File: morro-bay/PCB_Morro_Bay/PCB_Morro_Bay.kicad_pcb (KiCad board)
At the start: 2 copper layers, 220 x 145.5 mm, 346 parts, among them J1 POWER, J10 5V_12_8, J11 5V_12_9, J12 5V_12_10, J13 5V_12_11, J14 5V_12_12, J15 5V_12_13, J16 5V_12_14, J17 10V_12_1, J18 10V_12_2, J19 10V_12_3, J2 CAN, J20 10V_12_4, J21 10V_12_5, J22 10V_12_6, J23 POWER_OUT, J24 5V_16_1, J25 5V_16_2, J26 5V_16_3, J27 5V_16_4, J28 10V_16_1, J29 10V_16_2, J3 5V_12_1, J30 10V_16_3, J31 10V_16_4, J32 5V_16_5, J33 5V_16_6, J34 5V_16_7, J35 5V_16_8, J36 SWD, J37 GPIO, J38 USB_B, J39 ESERCOM, J4 5V_12_2, J5 5V_12_3, J6 5V_12_4, J7 5V_12_5, J8 5V_12_6, J9 5V_12_7, SW1 INPUT_RANGE_SEL_1, SW2 INPUT_RANGE_SEL_2, SW3 RESET, SW4 INPUT_RANGE_SEL_3, U1 MCP2515-xSO, U10 LM2902, U11 LM2902, U12 LM2902, U13 V7805-2000R, U2 SN65HVD232, U26 ADS114S08BIPBSR, U3 AZ1117-3.3, U4 ATSAMD21J18A-AU, U5 LM2902, U6 LM2902, U7 LM2902, U8 LM2902, U9 LM2902, Y1 8MHz, Y2 30MHz, Y3 32.768kHz

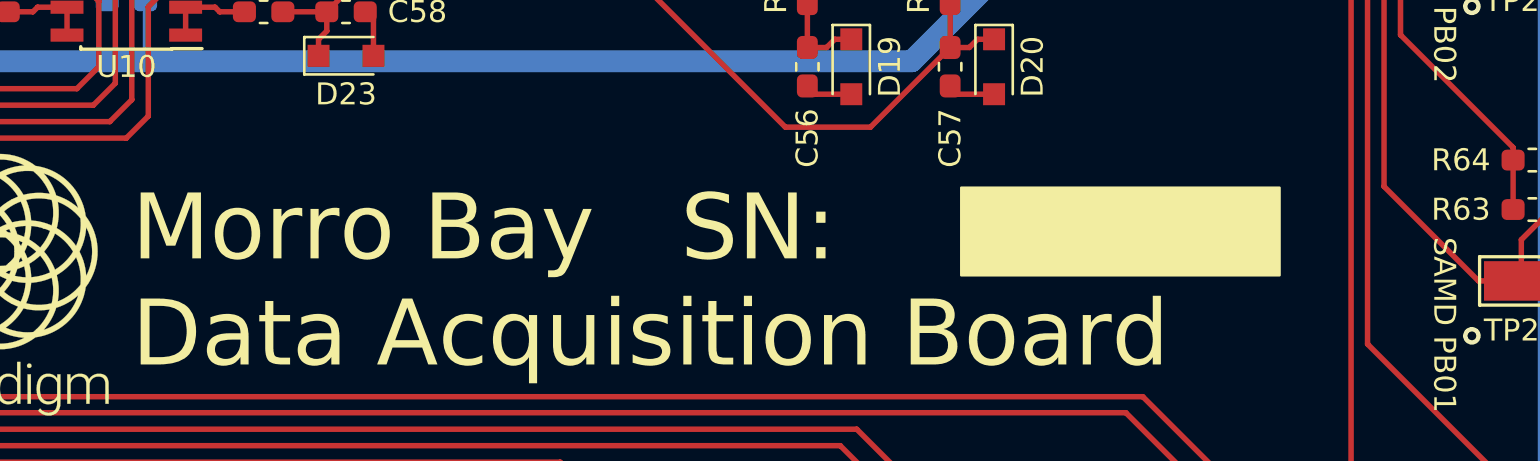
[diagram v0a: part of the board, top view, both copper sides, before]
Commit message: Export Gerbers
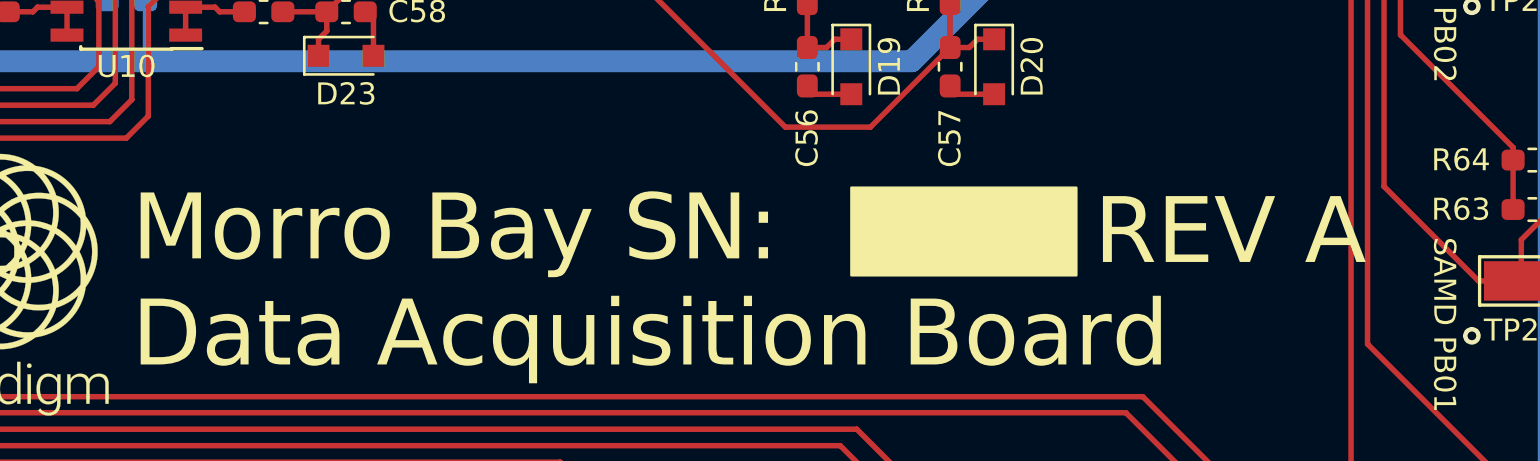
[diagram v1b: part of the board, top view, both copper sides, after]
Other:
- board text added: "REV A"
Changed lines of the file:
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@@
   (general
     (thickness 1.6)
-    (drawings 58)
+    (drawings 59)
     (tracks 2666)
     (zones 0)
@@
     (pad 4 smd rect (at 3.15 0.45) (size 1.2 0.6) (layers F.Cu F.Paste F.Mask))
   )
+  (gr_text "REV A" (at 291 168.75) (layer F.SilkS)
+    (effects (font (size 3 3) (thickness 0.3)))
+  )
   (gr_text "Copyright Paradigm Hyperloop, 2020\nAll Rights Reserved" (at 234.5 89.25) (layer F.SilkS)
     (effects (font (size 2 2) (thickness 0.3)) (justify left))
@@
     (arrow2b (pts (xy 101.25 44.25) (xy 102.376504 43.663579)))
   )
-  (gr_poly (pts (xy 278.75 170.75) (xy 293.25 170.75) (xy 293.25 166.75) (xy 278.75 166.75)) (layer F.SilkS) (width 0.1))
-  (gr_text "Morro Bay   SN:\nData Acquisition Board" (at 241 171) (layer F.SilkS)
+  (gr_poly (pts (xy 273.75 170.75) (xy 284 170.75) (xy 284 166.75) (xy 273.75 166.75)) (layer F.SilkS) (width 0.1))
+  (gr_text "Morro Bay SN:\nData Acquisition Board" (at 241 171) (layer F.SilkS)
     (effects (font (size 3 3) (thickness 0.3)) (justify left))
   )
